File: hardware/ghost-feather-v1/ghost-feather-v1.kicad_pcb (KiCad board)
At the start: 4 copper layers, 106.6 x 106.7 mm, 72 parts, among them J1 Conn_ARM_SWD_TagConnect_TC2030, J2 USB_C_Receptacle_USB2.0, J3 Conn_01x03, J4 Conn_01x03, J5 Conn_01x03, J6 Conn_01x03, J7 Conn_01x08, Q1 BSS138, Q2 BSS138, Q3 BSS138, Q4 BSS138, SW2 BOOT0, U1 STM32F722RETx, U2 BMI270, U3 USBLC6-2SC6_MOD, U4 MPM3610, U5 MPM3610, X1 16MHz, X2 32kHz768

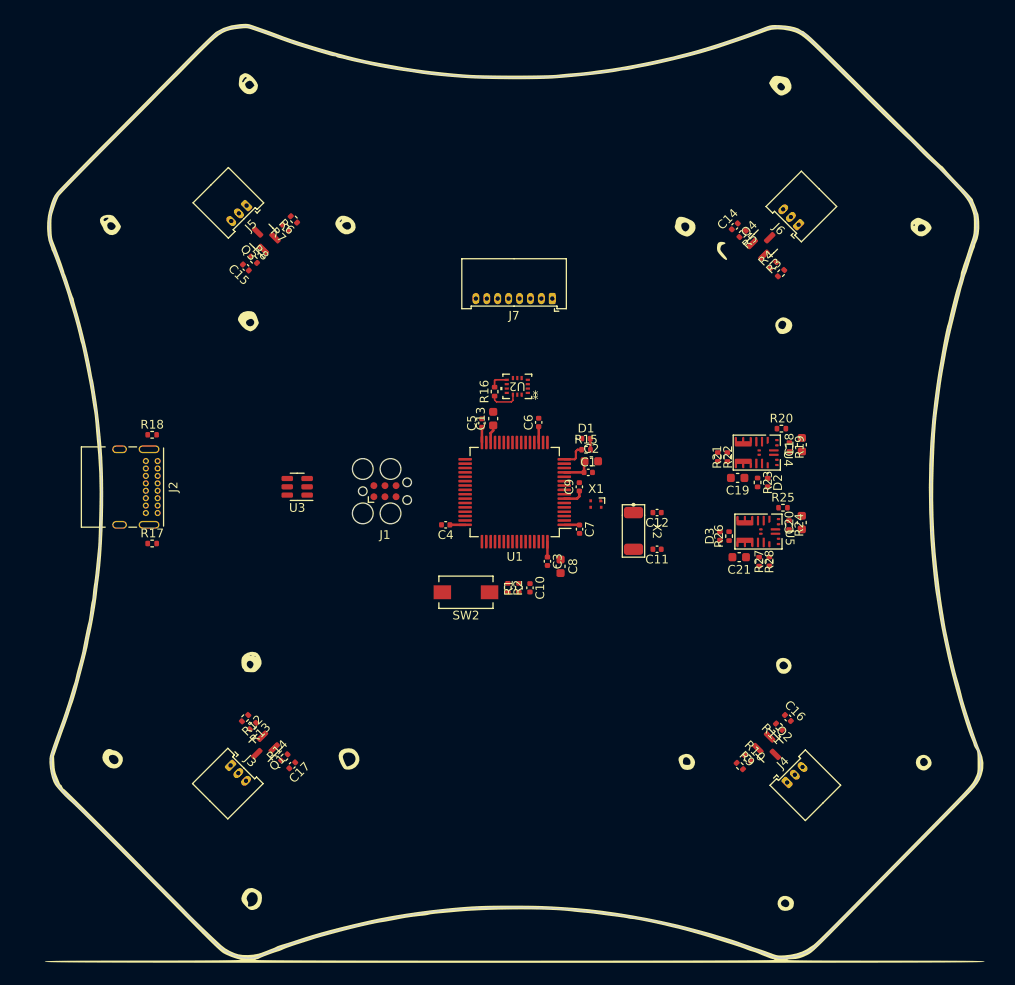
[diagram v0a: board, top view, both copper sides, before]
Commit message: feat: PCB routing #1
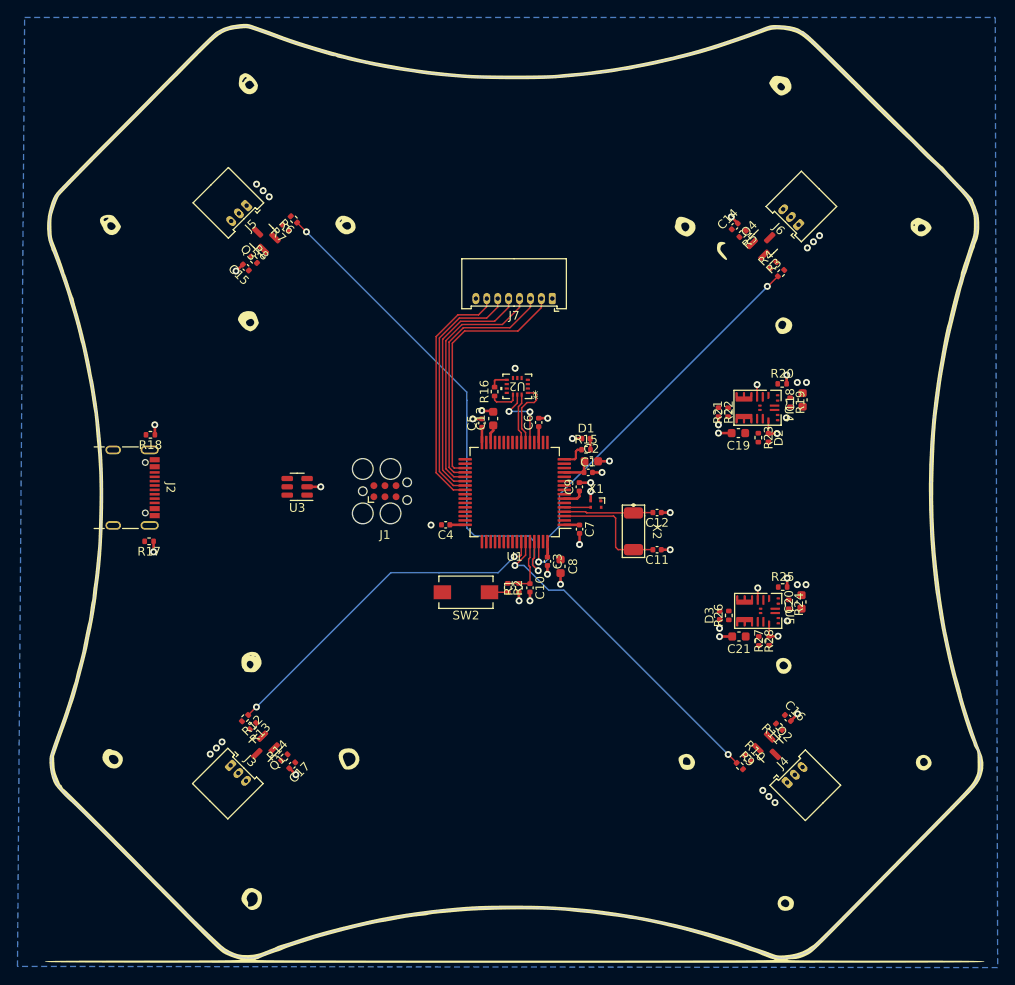
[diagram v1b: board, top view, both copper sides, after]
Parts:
- J2: footprint Connector_USB:USB_C_Receptacle_GCT_USB4085 -> Connector_USB:USB_C_Receptacle_GCT_USB4105-xx-A_16P_TopMnt_Horizontal
- moved R27 9.08 mm to (171.6, 108.9)
- moved C20 9.08 mm to (175.3, 104.5)
- moved C21 9.08 mm to (168.2, 108.4)
- moved D3 9.08 mm to (166.0, 106.0)
- moved R24 9.08 mm to (173.9, 104.8)
- moved R25 9.08 mm to (173.2, 102.8)
- moved R26 9.08 mm to (167.0, 106.0)
- moved R28 9.08 mm to (170.5, 108.9)
- moved U5 9.08 mm to (170.1, 105.5)
- moved C18 5.13 mm to (175.5, 81.3)
- moved C19 5.13 mm to (168.1, 85.2)
- moved D2 5.13 mm to (171.6, 85.7)
- moved R19 5.13 mm to (174.0, 81.6)
- moved R20 5.13 mm to (173.1, 79.5)
- moved R21 5.13 mm to (166.9, 82.8)
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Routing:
- net /ESC2: track 0.00 -> 58.8 mm, vias 0 -> 2
- net /ESC3: track 0.00 -> 46.9 mm, vias 0 -> 2
- net /ESC0: track 0.00 -> 40.4 mm, vias 0 -> 2
- net GND: track 0.00 -> 39.0 mm, vias 0 -> 52
- net /ESC1: track 0.00 -> 38.0 mm, vias 0 -> 2
- net /RF_CH0: track 0.00 -> 28.5 mm
- net /RF_CH1: track 0.00 -> 28.4 mm
- net /RF_CH2: track 0.00 -> 28.3 mm
- net /RF_CH3: track 0.00 -> 28.2 mm
- net /RF_CH4: track 0.00 -> 28.0 mm
- net /RF_CH5: track 0.00 -> 27.9 mm
- net /OSC32_IN: track 0.00 -> 13.7 mm
- net /OSC32_OUT: track 0.00 -> 10.2 mm
- net /SPI1_SCK: track 0.00 -> 8.24 mm, vias 0 -> 2
- net /SPI1_MISO: track 0.00 -> 7.90 mm
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- added copper zone on B.Cu, net GND
